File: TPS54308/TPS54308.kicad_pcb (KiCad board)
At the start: 2 copper layers, 25.4 x 12.7 mm, 12 parts, among them P1 CONN_01X02, P2 CONN_01X04, U1 TPS54308DDC

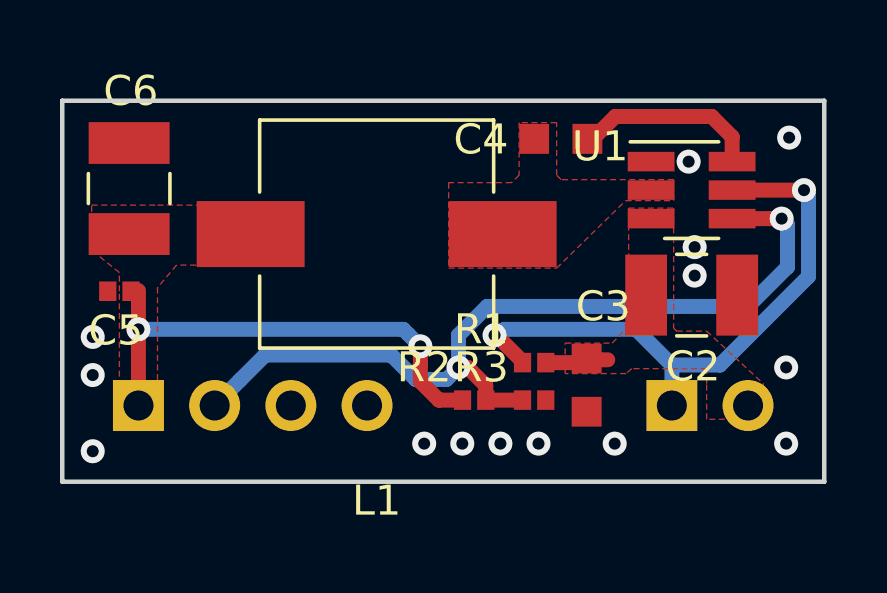
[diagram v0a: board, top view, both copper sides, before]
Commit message: Ready for prototyping
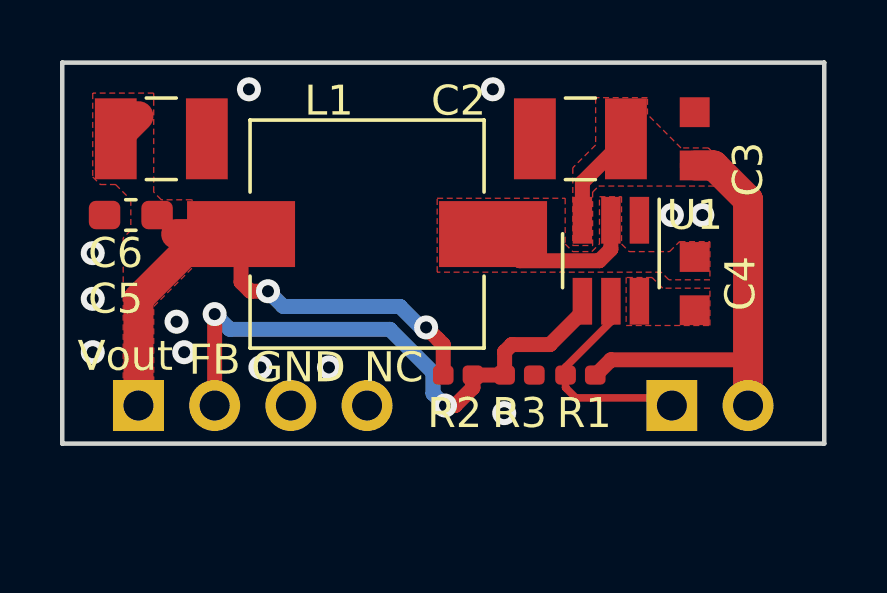
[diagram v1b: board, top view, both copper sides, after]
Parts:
- added REF**: OSHW-Logo2_7.3x6mm_SilkScreen, Symbol:OSHW-Logo2_7.3x6mm_SilkScreen, B.Cu at (118.0, 98.9)
- added REF**: KiCad-Logo2_5mm_SilkScreen, Symbol:KiCad-Logo2_5mm_SilkScreen, B.Cu at (108.2, 98.6)
- C5: footprint Capacitor_SMD:C_0402_1005Metric -> Capacitor_SMD:C_0603_1608Metric_Pad1.05x0.95mm_HandSolder
- L1: footprint Inductor_SMD:L_Wuerth_WE-PD-Typ-M-Typ-S_Handsoldering -> volatiles:L_Wuerth_WE-PD-Typ-M-Typ-S_Handsoldering
- R1, R2, R3: footprint Resistor_SMD:R_0402_1005Metric -> volatiles:R_0402_1005Metric_Handsolder
- moved C3 8.97 mm to (117.6, 97.8), turned to 90 degrees
- moved C4 6.57 mm to (117.6, 102.6), turned to 90 degrees
- moved C2 6.39 mm to (113.8, 97.8), turned to 180 degrees
- moved U1 3.58 mm to (114.8, 101.9), turned to 270 degrees
- moved C5 2.57 mm to (98.8, 100.3)
- moved C6 1.97 mm to (99.8, 97.8), turned to 0 degrees
- moved R1 1.60 mm to (113.8, 105.7)
- moved R2 0.99 mm to (109.7, 105.7)
- moved R3 0.97 mm to (111.8, 105.7)
- moved L1 0.32 mm to (106.7, 101.0)
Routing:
- net VIN: track 2.49 -> 18.0 mm
- net EN: track 20.3 -> 7.30 mm, vias 2 -> 0
- net FB: track 28.8 -> 19.3 mm
- net BOOT: track 6.24 -> 0.00 mm
- net SW: track 0.00 -> 5.42 mm
- net VOUT: track 16.5 -> 21.3 mm
- net GND: vias 14 -> 12
- added copper zone on F.Cu, net BOOT
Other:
- board text added: "FB"
- board text added: "GND"
- board text added: "NC"
- board text added: "StepDown 5-25V in 5V out (adj)"
- board text added: "Vout"
- board text added: "https://github.com/FHdB"
